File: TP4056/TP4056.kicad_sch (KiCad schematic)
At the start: 5 parts, among them J1 USB_B_Micro, U1 TP4056-42-ESOP8, U2 DW01A

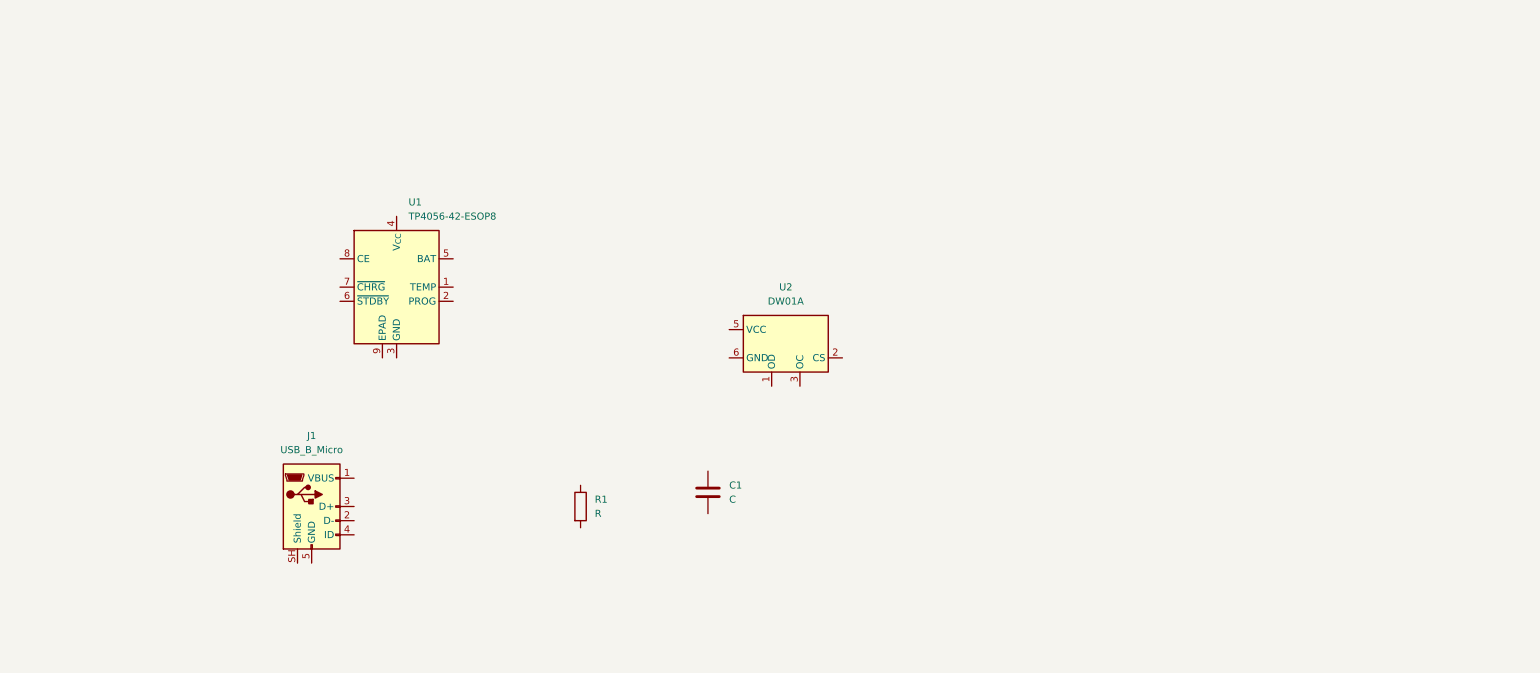
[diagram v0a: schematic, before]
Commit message: schematics completed
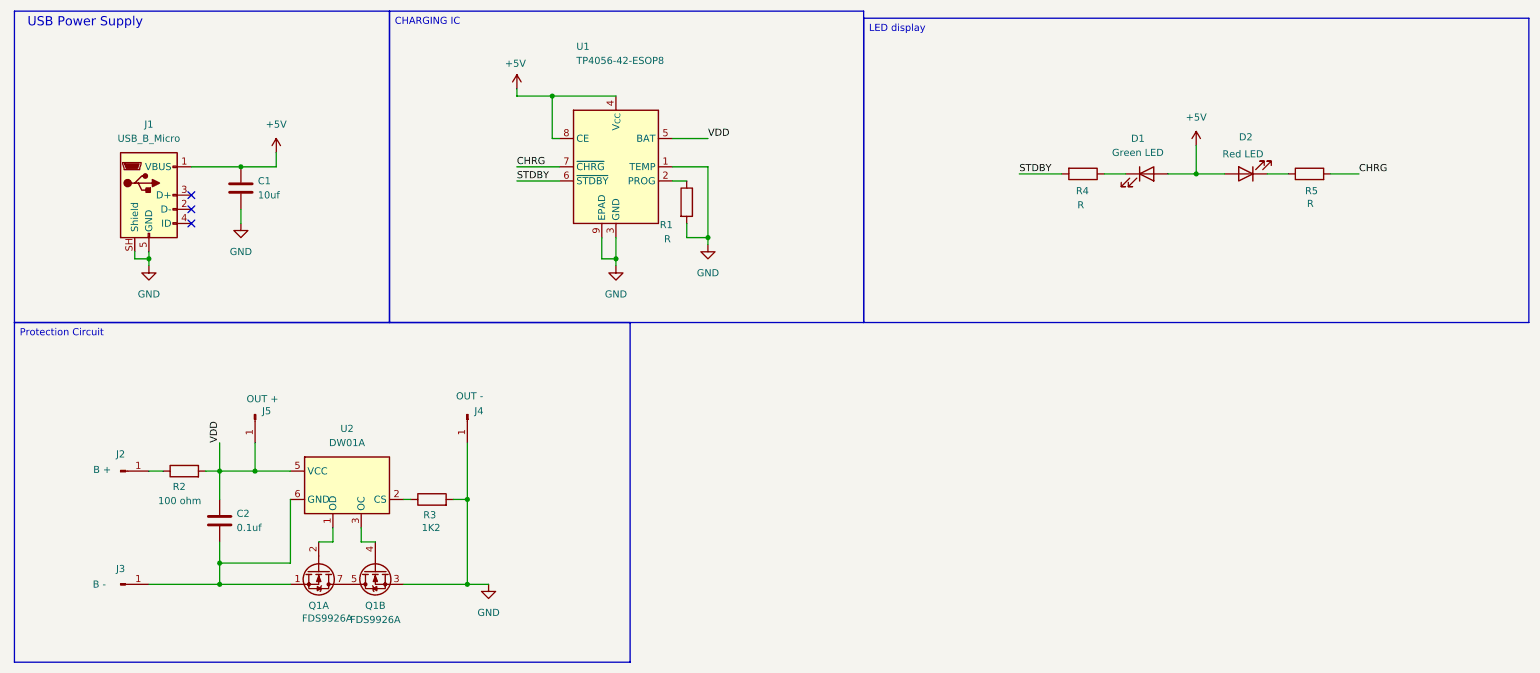
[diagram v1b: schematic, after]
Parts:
- added C2: 0.1uf, symbol Device:C
- added D1: Green LED, symbol Device:LED
- added D2: Red LED, symbol Device:LED
- added J2: B +, symbol Connector:Conn_01x01_Pin
- added J3: B -, symbol Connector:Conn_01x01_Pin
- added J4: OUT -, symbol Connector:Conn_01x01_Pin
- added J5: OUT +, symbol Connector:Conn_01x01_Pin
- added Q1: FDS9926A, Package_SO:SOIC-8_3.9x4.9mm_P1.27mm, symbol Transistor_FET:FDS9926A
- added R2: 100 ohm, symbol Device:R
- added R3: 1K2, symbol Device:R
- added R4, R5: R, symbol Device:R
- C1: value C -> 10uf
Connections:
- net at U2.1 (OD): now also Q1.2 (G1)
- net at U2.2 (CS): now also R3.1
- net at U2.3 (OC): now also Q1.4 (G2)
- net VDD: now reaches U2.5 (VCC)
- net VDD: now also U1.5 (BAT), C2.1, J5.1 (Pin_1), R2.2
- net at U2.6 (GND): now also C2.2, J3.1 (Pin_1), Q1.1 (S1)
- net +5V: now reaches J1.1 (VBUS)
- net +5V: now also C1.1, U1.4 (V_{CC}), U1.8 (CE), D1.2 (A), D2.2 (A)
- net GND: now reaches J1.5 (GND)
- net GND: now also C1.2, J1.SH (Shield), R1.2, U1.1 (TEMP), U1.3 (GND), U1.9 (EPAD), J4.1 (Pin_1), Q1.3 (S2), R3.2
- net at R1.1: now also U1.2 (PROG)
- net STDBY: now reaches U1.6 (~{STDBY})
- net STDBY: now also R4.2
- net CHRG: now reaches U1.7 (~{CHRG})
- net CHRG: now also R5.2
- new net: Q1.5 (D2), Q1.6 (D2), Q1.7 (D1), Q1.8 (D1)
- new net: J2.1 (Pin_1), R2.1
- new net: D2.1 (K), R5.1
- new net: D1.1 (K), R4.1
- no-connect marks 0 -> 3
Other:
- note added: "USB Power Supply"
- moved on the sheet: C1, J1, R1, U1, U2
